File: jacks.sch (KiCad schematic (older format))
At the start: 71 parts, among them J601 PJ301CM, J602 PJ301CM, J603 PJ301BM, J604 PJ301BM, J605 PJ301BM, J606 PJ301BM, J607 PJ301BM, J608 PJ301BM, J609 PJ301BM, J610 PJ301BM, J611 PJ301BM, J612 PJ301BM, J613 PJ301BM, J614 PJ301BM, J615 PJ301BM, J616 PJ301BM, J617 PJ301BM, J618 PJ301BM, J619 PJ301BM, J620 PJ301BM, J621 PJ301BM, J622 PJ301BM, J623 PJ301BM, J624 PJ301BM, J625 PJ301BM, J626 PJ301BM, Q601 MMBT3904, Q602 MMBT3904, Q603 MMBT3904, Q604 MMBT3904, U601 TL074, U602 6N137

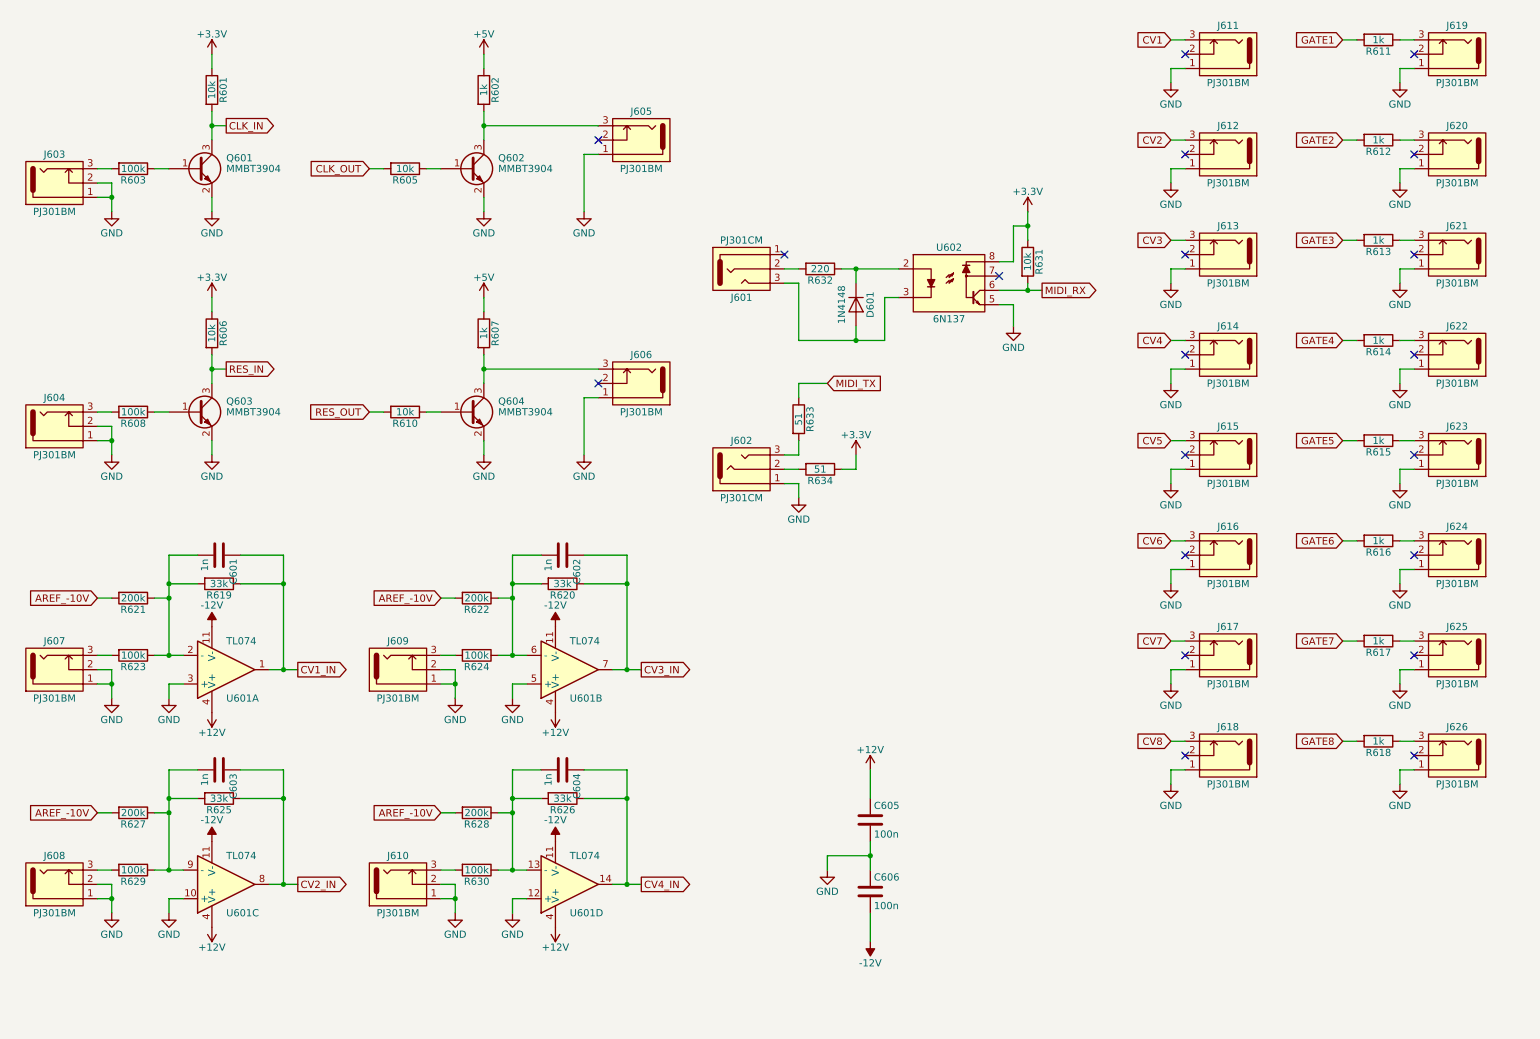
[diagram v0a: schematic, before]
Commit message: work in progress
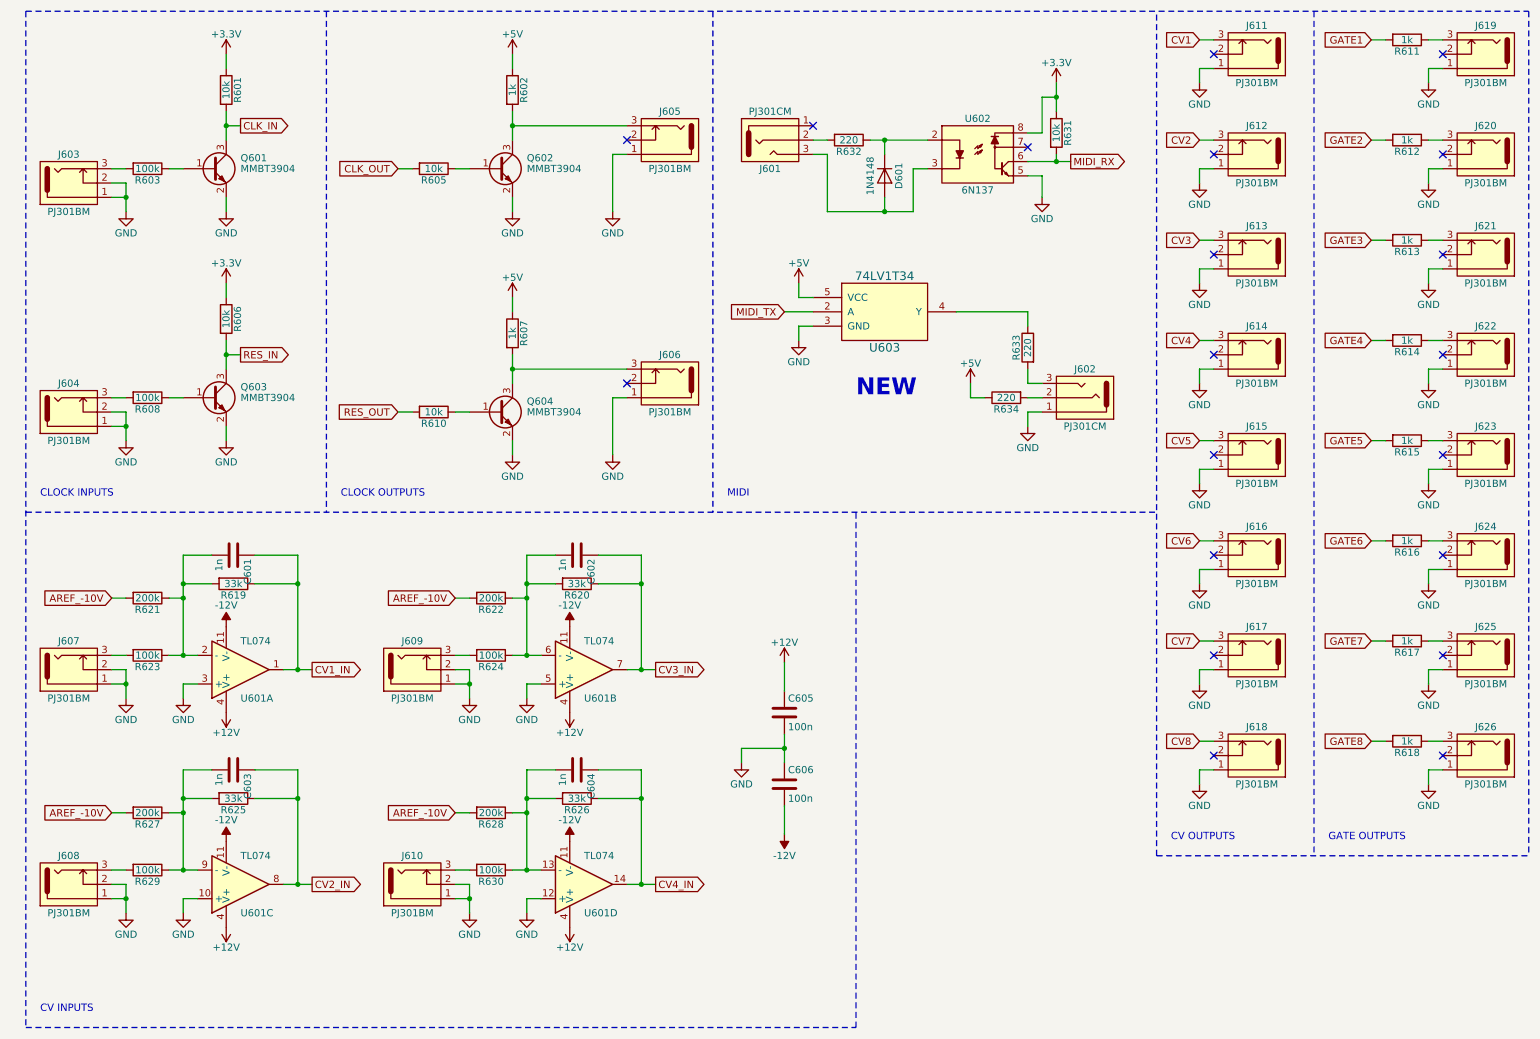
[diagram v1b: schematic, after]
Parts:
- added U603: 74LV1T34, symbol 74LV1T34
- C601, C602, C603, C604, C605, C606: footprint Capacitors_SMD:C_0603 -> Capacitors_SMD:C_0603_HandSoldering
- R601, R602, R603, R605, R606, R607, R608, R610, R611, R612, R613, R614, R615, R616, R617, R618, R619, R620, R621, R622, R623, R624, R625, R626, R627, R628, R629, R630, R631, R632: footprint Resistors_SMD:R_0603 -> Resistors_SMD:R_0603_HandSoldering
- R633, R634: value 51 -> 220; footprint Resistors_SMD:R_0603 -> Resistors_SMD:R_0603_HandSoldering
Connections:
- net +3V3: no longer R634.1
- net +5V: now also R634.1, U603.5 (VCC)
- net GND: now also U603.3 (GND)
- net MIDI_TX: now also U603.2 (A); no longer R633.1
- new net: R633.1, U603.4 (Y)
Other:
- note added: "CLOCK INPUTS"
- note added: "CLOCK OUTPUTS"
- note added: "CV INPUTS"
- note added: "CV OUTPUTS"
- note added: "GATE OUTPUTS"
- note added: "MIDI"
- note added: "NEW"
- moved on the sheet: C601, C602, C603, C604, C605, C606, D601, J601, J602, J603, J604, J605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
